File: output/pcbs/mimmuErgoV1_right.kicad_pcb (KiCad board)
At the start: 2 copper layers, 144.7 x 96.9 mm, 47 parts

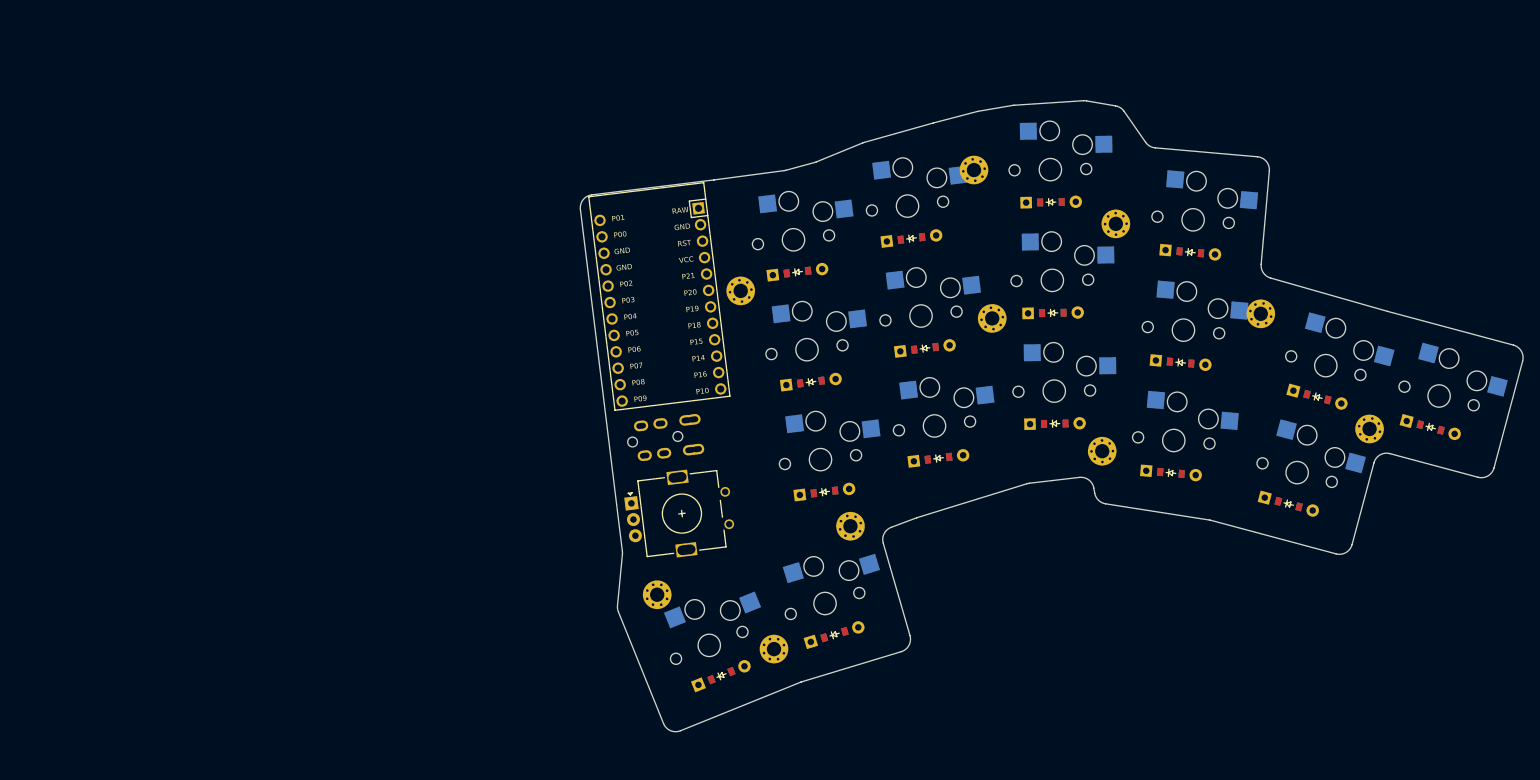
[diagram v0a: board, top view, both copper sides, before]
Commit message: Add files via upload
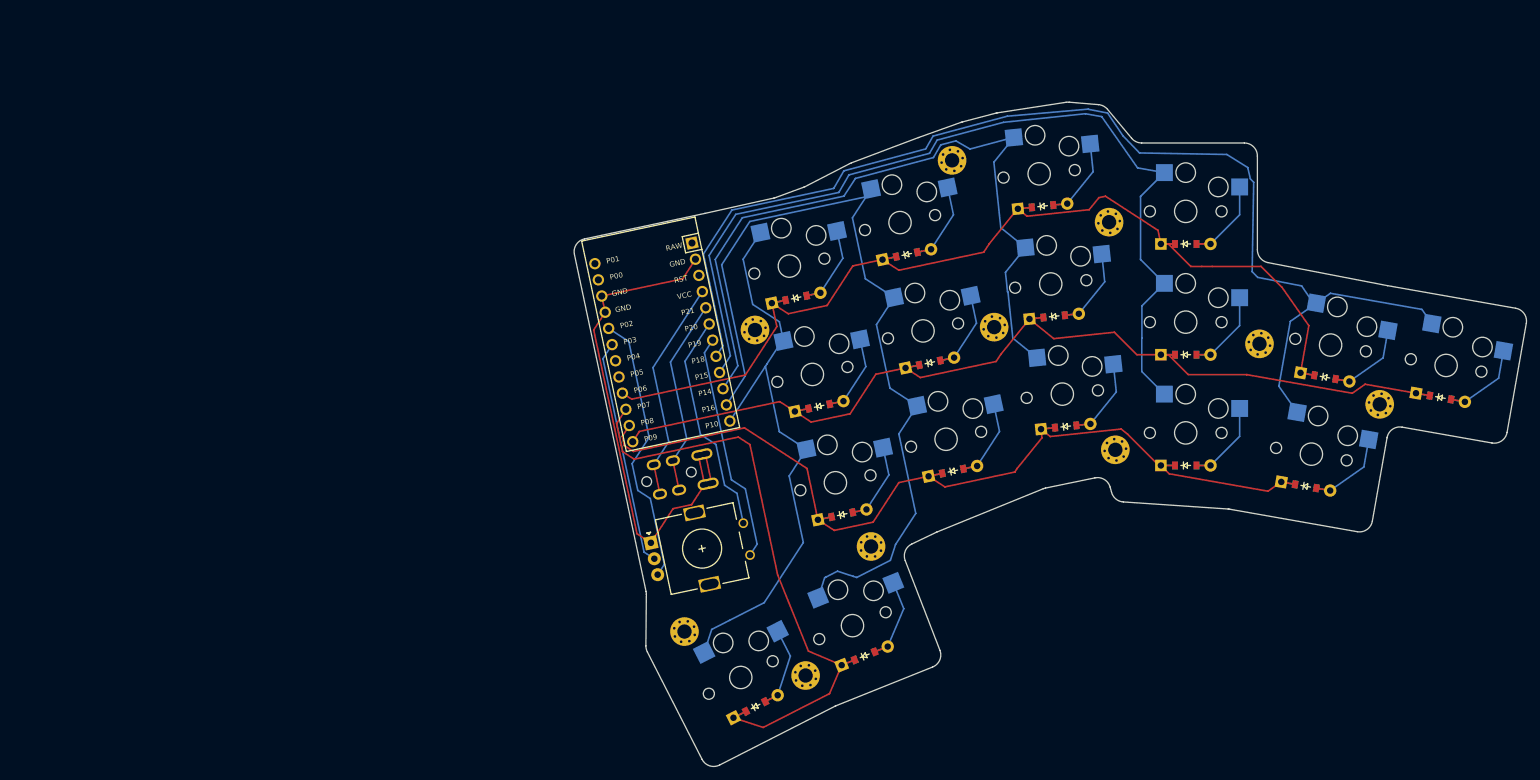
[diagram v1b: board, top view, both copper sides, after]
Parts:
- moved D17 7.07 mm to (261.5, 216.1), turned to 27 degrees
- moved _4 7.04 mm to (250.6, 204.6), turned to 27 degrees
- moved S17 6.91 mm to (259.3, 211.7), turned to 27 degrees
- moved TRRS1 6.55 mm to (242.8, 179.7), turned to 102 degrees
- moved _3 6.39 mm to (261.5, 158.4), turned to 12 degrees
- moved _5 6.33 mm to (269.2, 211.4), turned to 27 degrees
- moved ROT1 6.19 mm to (253.5, 191.9), turned to 12 degrees
- moved MCU1 5.79 mm to (247.2, 160.3), turned to -78 degrees
- moved D16 5.65 mm to (278.3, 208.4), turned to 22 degrees
- moved S16 5.41 mm to (276.4, 203.7), turned to 22 degrees
- moved D3 4.83 mm to (366.7, 168.7), turned to -10 degrees
- moved S3 4.81 mm to (367.5, 163.8), turned to -10 degrees
- moved _10 4.61 mm to (338.9, 160.5), turned to -10 degrees
- moved _6 4.43 mm to (279.3, 191.6), turned to 22 degrees
- moved D13 4.41 mm to (274.8, 186.7), turned to 12 degrees
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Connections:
- D2 pad 1: P9 -> P6
- D3 pad 1: P6 -> P9
- ROT1 pad B: P3 -> P2
- ROT1 pad C: P2 -> P3
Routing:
- net P18: track 0.00 -> 179.0 mm
- net P6: track 0.00 -> 161.9 mm
- net P9: track 0.00 -> 156.1 mm
- net P8: track 0.00 -> 147.5 mm
- net P15: track 0.00 -> 140.2 mm
- net P16: track 0.00 -> 130.5 mm
- net P14: track 0.00 -> 113.9 mm
- net P7: track 0.00 -> 95.8 mm
- net P10: track 0.00 -> 89.1 mm
- net GND: track 0.00 -> 80.8 mm
- net P2: track 0.00 -> 42.2 mm
- net P19: track 0.00 -> 35.5 mm
- net P3: track 0.00 -> 35.0 mm
- net P20: track 0.00 -> 34.5 mm
- net VCC: track 0.00 -> 34.4 mm
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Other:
- board size 144.7 x 96.9 mm -> 146.2 x 102 mm
- net class Default removed

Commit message: finalize
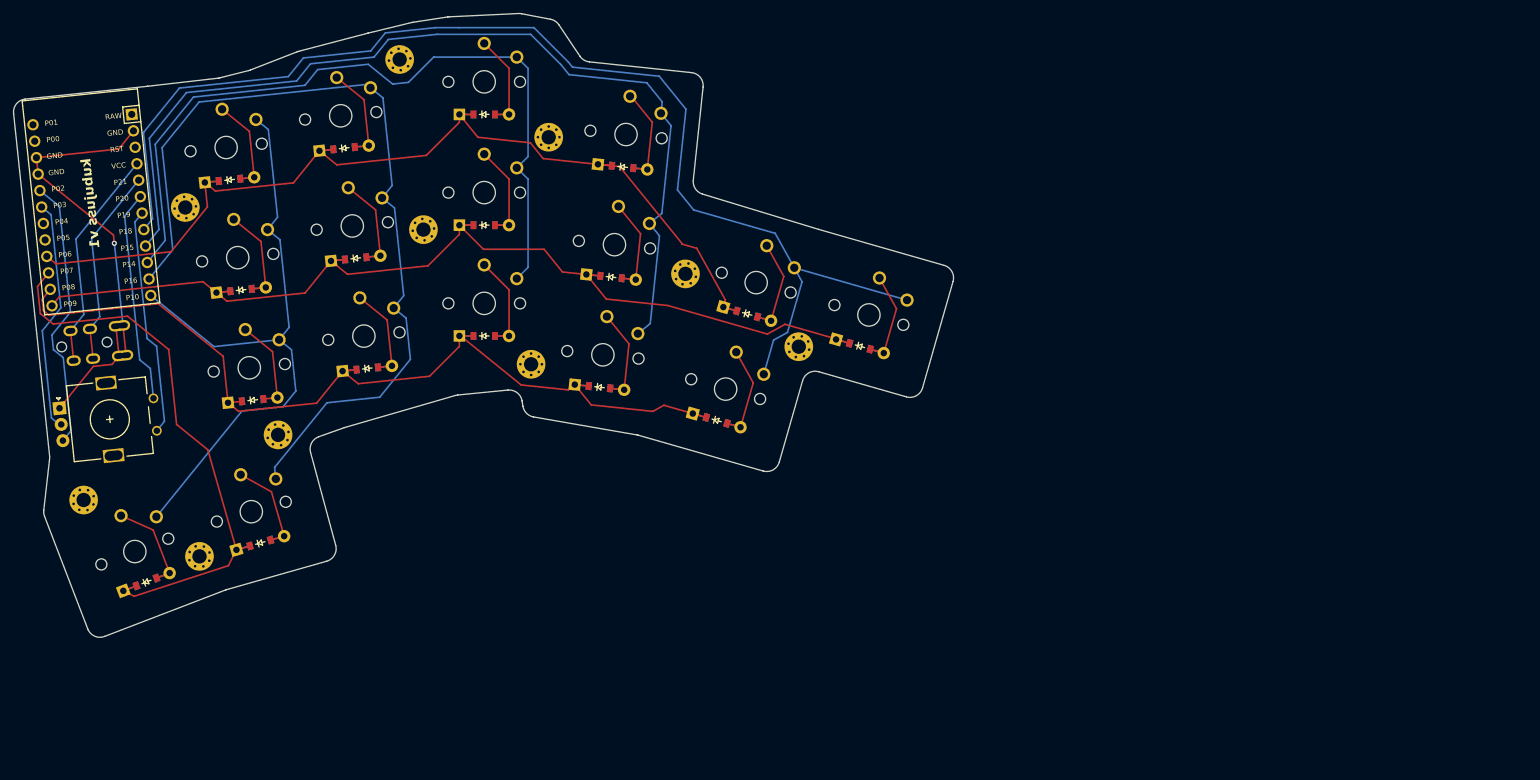
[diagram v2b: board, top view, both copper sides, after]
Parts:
- moved D17 95.4 mm to (168.1, 197.0), turned to 21 degrees
- moved S17 95.0 mm to (166.3, 192.4), turned to 21 degrees
- moved _5 94.8 mm to (176.2, 193.1), turned to 21 degrees
- moved _4 94.4 mm to (158.4, 184.4), turned to 21 degrees
- moved D16 94.4 mm to (185.5, 191.0), turned to 16 degrees
- moved S16 93.9 mm to (184.1, 186.2), turned to 16 degrees
- moved ROT1 93.0 mm to (162.5, 172.1), turned to 6 degrees
- moved _6 92.6 mm to (188.3, 174.5), turned to 16 degrees
- moved D13 92.2 mm to (184.4, 169.1), turned to 6 degrees
- moved TRRS1 92.0 mm to (153.2, 158.8), turned to 96 degrees
- moved S13 91.7 mm to (183.8, 164.2), turned to 6 degrees
- moved D10 91.2 mm to (201.9, 164.3), turned to 6 degrees
- moved D1 91.0 mm to (255.6, 172.2), turned to -16 degrees
- moved D4 90.8 mm to (237.6, 167.1), turned to -6 degrees
- moved S10 90.8 mm to (201.4, 159.3), turned to 6 degrees
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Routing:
- net P10: track 89.1 -> 98.5 mm
- net GND: track 80.8 -> 71.9 mm, vias 0 -> 1
- net P6: track 161.9 -> 155.3 mm
- net P14: track 113.9 -> 119.0 mm
- net P15: track 140.2 -> 144.9 mm
- net P7: track 95.8 -> 91.2 mm
- net P8: track 147.5 -> 144.7 mm
- net P18: track 179.0 -> 181.8 mm
- net P16: track 130.5 -> 133.0 mm
- net mirror_ring_top: track 14.9 -> 16.9 mm
- net mirror_space_cluster: track 14.9 -> 16.8 mm
- net mirror_middle_top: track 14.9 -> 16.8 mm
- net mirror_pinkie_top: track 14.9 -> 16.8 mm
- net mirror_index_top: track 14.9 -> 16.8 mm
- net mirror_ring_bottom: track 14.9 -> 16.8 mm
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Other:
- board size 146.2 x 102 mm -> 144.3 x 95.7 mm
- board text added: "kubujuss v1"
